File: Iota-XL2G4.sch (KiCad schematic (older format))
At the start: 34 parts, among them J1 u.fl, U1 STM32G071EBY6TR, U2 NCP160, U3 SX1280, U4 2450FM07D0034T, Y1 52M

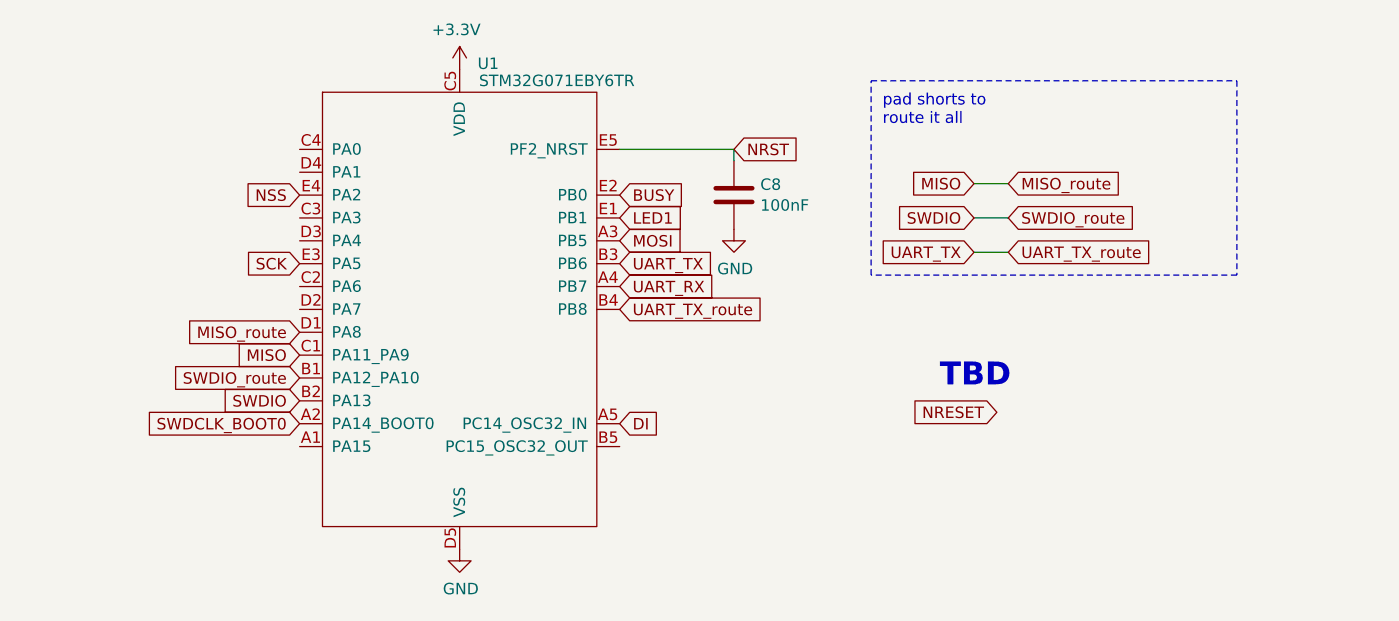
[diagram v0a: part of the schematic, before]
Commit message: general update
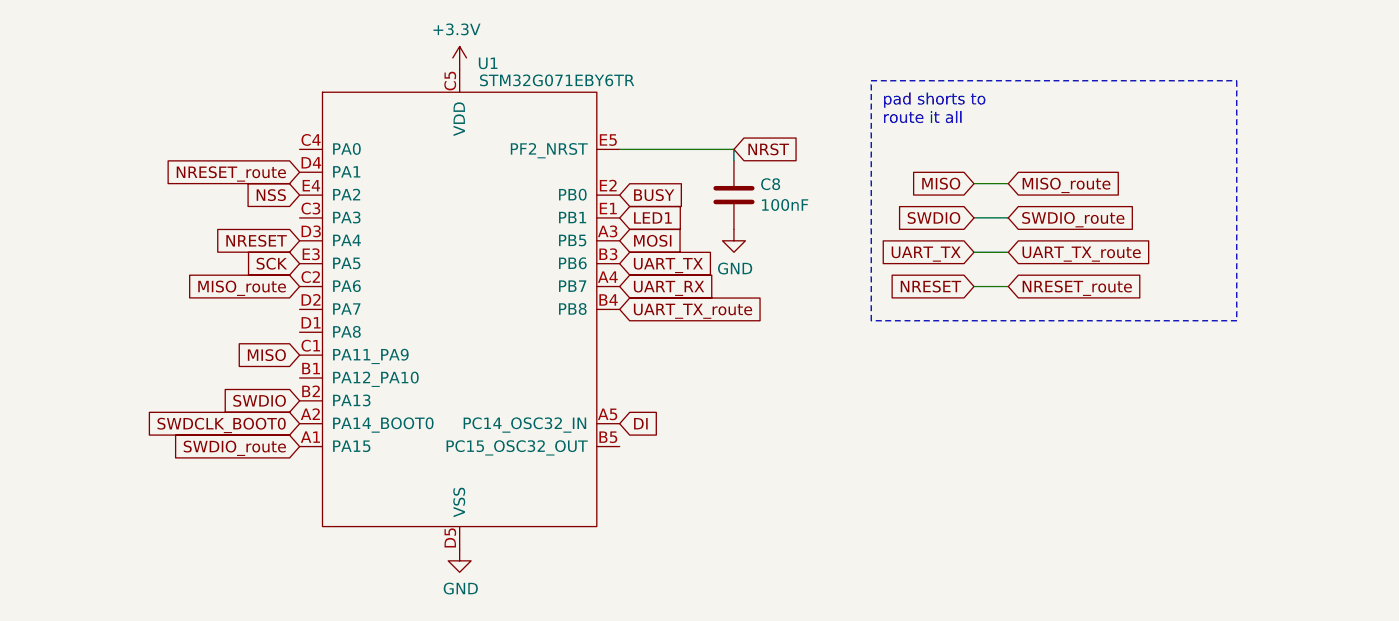
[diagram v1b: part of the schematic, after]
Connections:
- net MISO: now also U1.C2 (PA6); no longer U1.D1 (PA8)
- net NRESET: now also U1.D3 (PA4), U1.D4 (PA1)
- net SWDIO: now also U1.A1 (PA15); no longer U1.B1 (PA12_PA10)
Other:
- note removed: "TBD"
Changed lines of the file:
@@
 Text GLabel 1800 1400 0    50   Input ~ 0
 NSS
-Text GLabel 1800 2200 0    50   Input ~ 0
+Text GLabel 1800 2500 0    50   Input ~ 0
 SWDIO_route
 Text GLabel 3200 1900 2    50   Input ~ 0
@@
 Text GLabel 3200 1400 2    50   Input ~ 0
 BUSY
-Text GLabel 1800 2000 0    50   Input ~ 0
+Text GLabel 1800 1800 0    50   Input ~ 0
 MISO_route
 Text GLabel 3200 1500 2    50   Input ~ 0
 LED1
-Text GLabel 4850 2350 0    50   Input ~ 0
+Text GLabel 1800 1600 0    50   Input ~ 0
 NRESET
 Wire Notes Line
 	4300 900  5900 900
 Wire Notes Line
-	5900 900  5900 1750
+	5900 900  5900 1950
 Wire Notes Line
-	5900 1750 4300 1750
+	5900 1950 4300 1950
 Wire Notes Line
-	4300 1750 4300 900
+	4300 1950 4300 900
 Text Notes 4350 1100 0    50   ~ 0
 pad shorts to\nroute it all
-Text Notes 4600 2250 0    100  ~ 20
-TBD
+Text GLabel 1800 1300 0    50   Input ~ 0
+NRESET_route
+Text GLabel 4750 1800 0    50   Input ~ 0
+NRESET
+Text GLabel 4900 1800 2    50   Input ~ 0
+NRESET_route
+Wire Wire Line
+	4750 1800 4900 1800
 $EndSCHEMATC
